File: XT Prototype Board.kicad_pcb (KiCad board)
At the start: 2 copper layers, 101.6 x 101.6 mm, 5 parts, among them J1 Bus_ISA_8bit, J2 Breakout

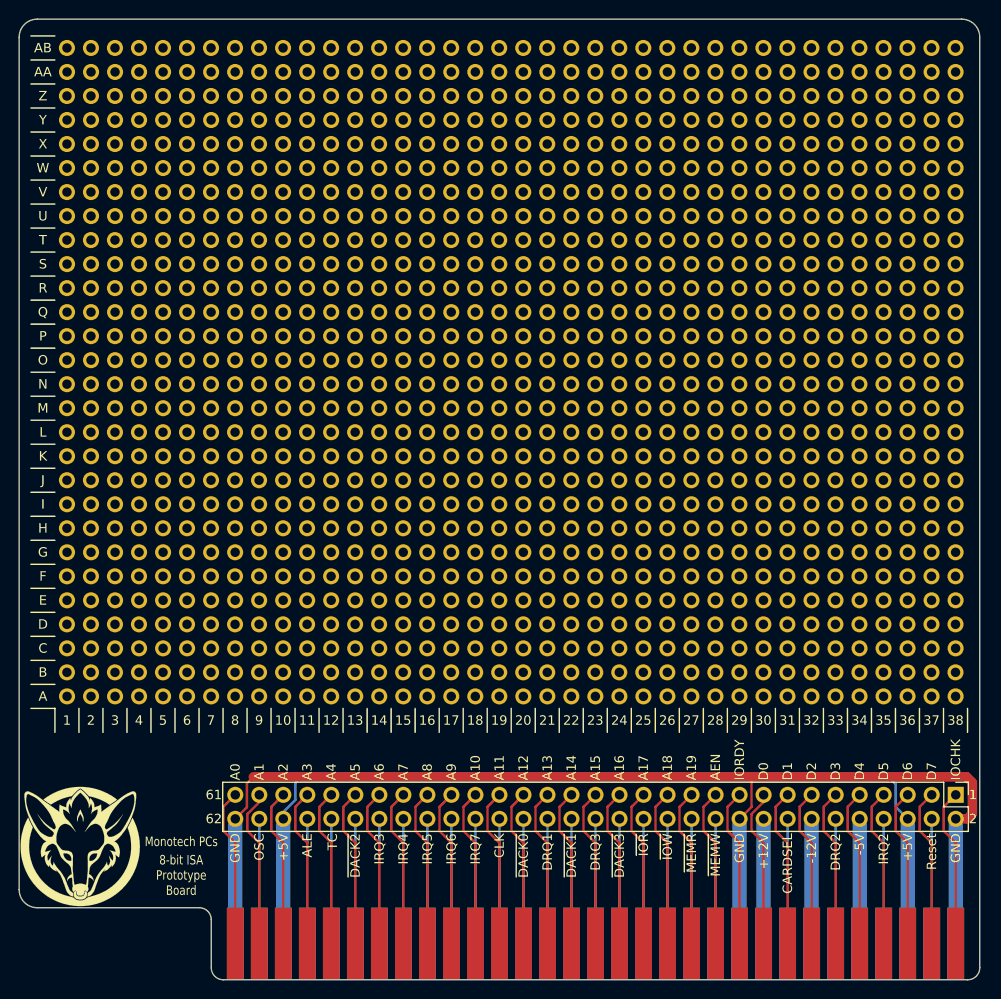
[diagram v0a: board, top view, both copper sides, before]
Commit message: updated to kicad 7.0
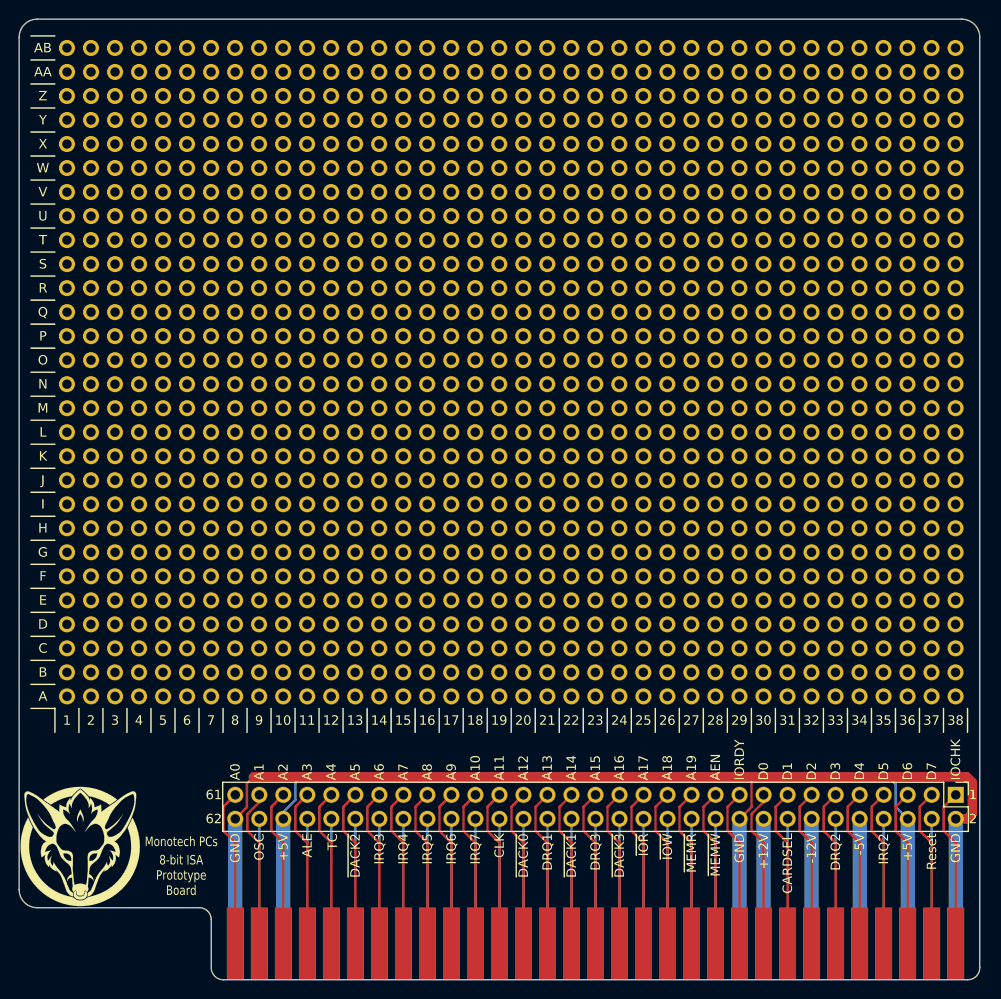
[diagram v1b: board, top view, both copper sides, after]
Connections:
- net ~DACK0 renamed ~{DACK0}
- net ~DACK1 renamed ~{DACK1}
- net ~DACK2 renamed ~{DACK2}
- net ~DACK3 renamed ~{DACK3}
- net ~IOR renamed ~{IOR}
- net ~IOW renamed ~{IOW}
- net ~MEMR renamed ~{MEMR}
- net ~MEMW renamed ~{MEMW}
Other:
- net class Default removed
- board text added: "~{DACK0}"
- board text added: "~{DACK1}"
- board text added: "~{DACK2}"
- board text added: "~{DACK3}"
- board text added: "~{IOR}"
- board text added: "~{IOW}"
- board text added: "~{MEMR}"
- board text added: "~{MEMW}"
- board text removed: "~DACK0"
- board text removed: "~DACK1"
- board text removed: "~DACK2"
- board text removed: "~DACK3"
- board text removed: "~IOR"
- board text removed: "~IOW"
- board text removed: "~MEMR"
- board text removed: "~MEMW"
